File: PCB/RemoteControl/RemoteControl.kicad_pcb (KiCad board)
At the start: 2 copper layers, 44 x 54.5 mm, 14 parts, among them J1 USB_C_Receptacle_USB2.0_14P, J2 Conn_02x05_Top_Bottom, J3 Conn_01x06, J4 Conn_01x03, SW1 SW_Push, U1 STM32L031K6Tx, U2 TC1262-33

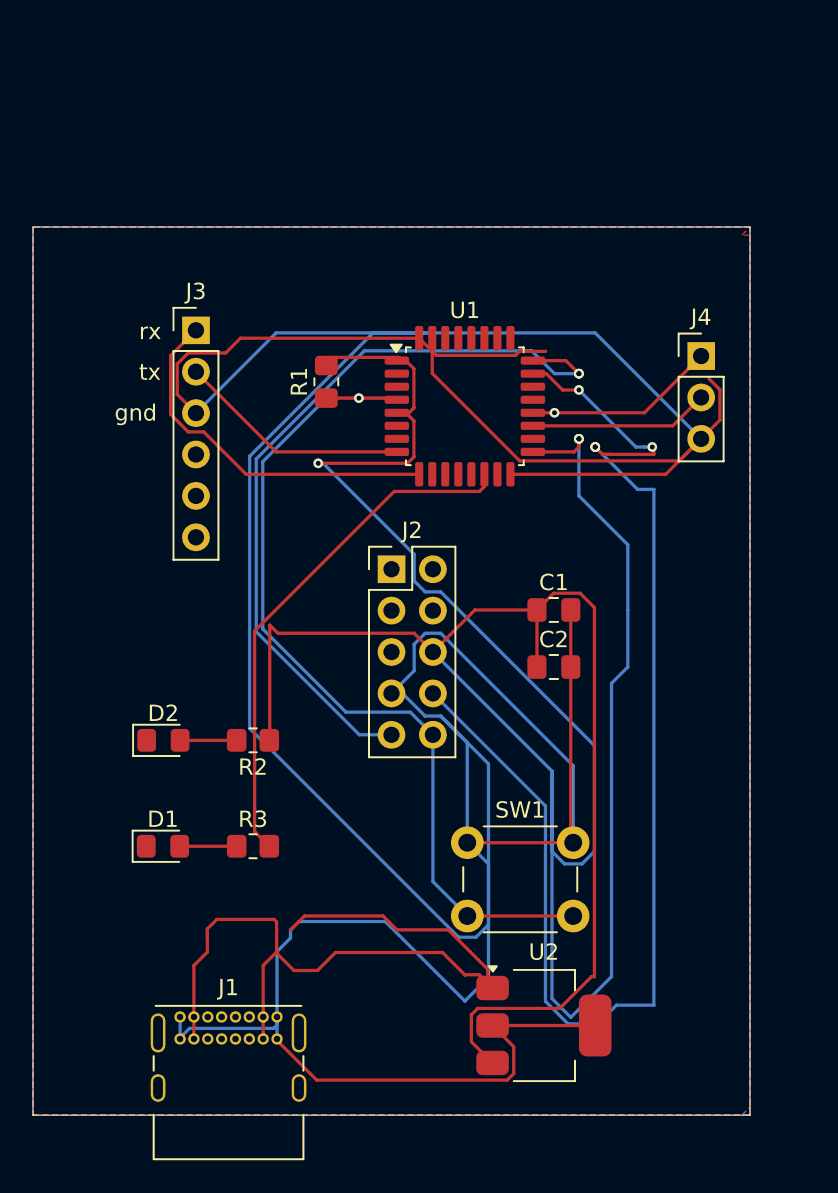
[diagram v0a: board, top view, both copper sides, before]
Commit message: push
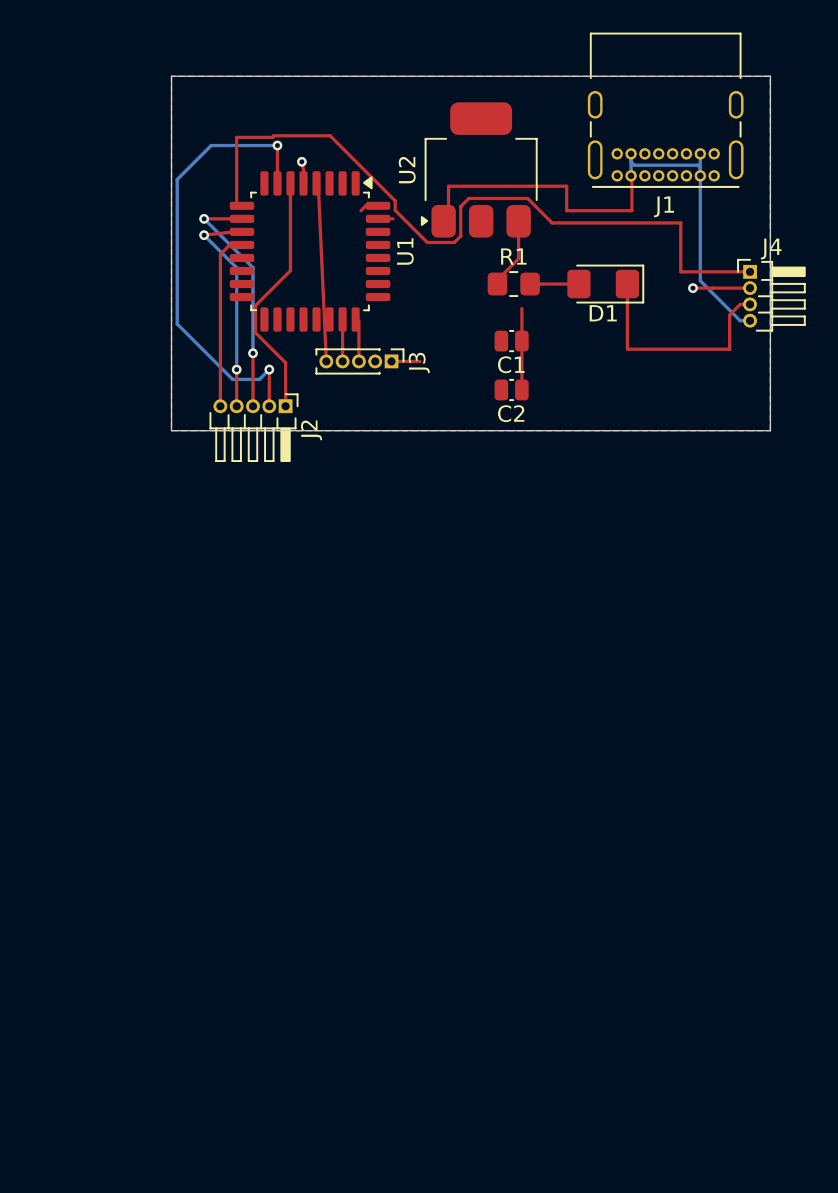
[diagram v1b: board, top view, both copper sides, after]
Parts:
- removed D2: LED, LED_SMD:LED_0805_2012Metric_Pad1.15x1.40mm_HandSolder
- removed R2, R3: 330, Resistor_SMD:R_0805_2012Metric_Pad1.20x1.40mm_HandSolder
- removed SW1: SW_Push, Button_Switch_THT:SW_PUSH_6mm_H4.3mm
- C1: value .1uf -> .1u; footprint Capacitor_SMD:C_0805_2012Metric_Pad1.18x1.45mm_HandSolder -> Capacitor_SMD:C_0504_1310Metric_Pad0.83x1.28mm_HandSolder
- C2: value 10uf -> 1; footprint Capacitor_SMD:C_0805_2012Metric_Pad1.18x1.45mm_HandSolder -> Capacitor_SMD:C_0504_1310Metric_Pad0.83x1.28mm_HandSolder
- D1: footprint LED_SMD:LED_0805_2012Metric_Pad1.15x1.40mm_HandSolder -> LED_SMD:LED_1206_3216Metric_Pad1.42x1.75mm_HandSolder
- J2: value Conn_02x05_Top_Bottom -> Conn_01x05_Socket; footprint Connector_PinHeader_2.54mm:PinHeader_2x05_P2.54mm_Vertical -> Connector_PinHeader_1.00mm:PinHeader_1x05_P1.00mm_Horizontal
- J3: value Conn_01x06 -> Conn_01x05_Pin; footprint Connector_PinHeader_2.54mm:PinHeader_1x06_P2.54mm_Vertical -> Connector_PinHeader_1.00mm:PinHeader_1x05_P1.00mm_Vertical
- J4: value Conn_01x03 -> Conn_01x04_Socket; footprint Connector_PinHeader_2.54mm:PinHeader_1x03_P2.54mm_Vertical -> Connector_PinHeader_1.00mm:PinHeader_1x04_P1.00mm_Horizontal
- R1: value 4.7k -> 270
- moved J1 61.1 mm to (66.3, 25.9), turned to 180 degrees
- moved U2 52.6 mm to (52.0, 25.5), turned to 90 degrees
- moved D1 43.8 mm to (59.5, 32.5), turned to 180 degrees
- moved C2 17.2 mm to (53.9, 39.0), turned to 180 degrees
- moved C1 16.7 mm to (53.9, 36.0), turned to 180 degrees
- moved U1 13.4 mm to (41.5, 30.5), turned to -90 degrees
- moved R1 13.0 mm to (54.0, 32.5), turned to 0 degrees
- moved J3 12.2 mm to (46.5, 37.2), turned to -90 degrees
- moved J2 11.9 mm to (40.0, 40.0), turned to -90 degrees
- moved J4 5.98 mm to (68.5, 31.8)
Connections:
- C1 pad 1: VAPP -> +3.3V
- C2 pad 1: VAPP -> +3.3V
- J2 pad 1: unconnected-(J2-Pin_1-Pad1) -> Finger1
- J2 pad 2: unconnected-(J2-Pin_2-Pad2) -> Finger2
- J2 pad 3: unconnected-(J2-Pin_3-Pad3) -> Finger3
- J2 pad 4: unconnected-(J2-Pin_4-Pad4) -> Finger4
- J2 pad 5: unconnected-(J2-Pin_5-Pad5) -> Finger5
- J3 pad 1: rx -> +3.3V
- J3 pad 2: tx -> GND
- J3 pad 3: GND -> SWSCLK
- J3 pad 4: unconnected-(J3-Pin_4-Pad4) -> SWDIO
- J3 pad 5: unconnected-(J3-Pin_5-Pad5) -> NRST
- J4 pad 1: SDA -> RX
- J4 pad 2: SCL -> TX
- R1 pad 1: NRST -> +3.3V
- R1 pad 2: VAPP -> Net-(D1-A)
- U1 pad 1: VAPP -> +3.3V
- U1 pad 10: unconnected-(U1-PA4-Pad10) -> Finger3
- U1 pad 11: unconnected-(U1-PA5-Pad11) -> Finger4
- U1 pad 12: unconnected-(U1-PA6-Pad12) -> Finger5
- U1 pad 14: Net-(U1-PB0) -> unconnected-(U1-PB0-Pad14)
- U1 pad 17: VAPP -> +3.3V
- U1 pad 19: SCL -> unconnected-(U1-PA9-Pad19)
- U1 pad 20: SDA -> unconnected-(U1-PA10-Pad20)
- U1 pad 23: TMS_SWDIO -> SWDIO
- U1 pad 24: TCK_SWCLK -> SWSCLK
- U1 pad 5: VAPP -> +3.3V
- U1 pad 6: unconnected-(U1-PA0-Pad6) -> Finger1
- U1 pad 7: unconnected-(U1-PA1-Pad7) -> Finger2
- U1 pad 8: tx -> TX
- U1 pad 9: rx -> RX
- U2 pad 3: VAPP -> +3.3V
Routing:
- net GND: track 286.6 -> 16.0 mm
- net VAPP: track 189.8 -> 0.00 mm, vias 3 -> 0
- net TMS_SWDIO: track 79.7 -> 0.00 mm, vias 4 -> 0
- net NRST: track 56.0 -> 0.00 mm, vias 1 -> 0
- net TCK_SWCLK: track 47.8 -> 0.00 mm, vias 2 -> 0
- net Net-(U1-PB0): track 32.1 -> 0.00 mm
- net +5V: track 49.4 -> 18.6 mm
- net RX: track 0.00 -> 30.9 mm
- net Finger2: track 0.00 -> 28.0 mm, vias 0 -> 2
- net rx: track 22.6 -> 0.00 mm
- net Finger1: track 0.00 -> 15.3 mm
- net tx: track 14.4 -> 0.00 mm
- net Finger3: track 0.00 -> 13.0 mm, vias 0 -> 2
- net SDA: track 11.8 -> 0.00 mm, vias 1 -> 0
- net Finger4: track 0.00 -> 11.6 mm, vias 0 -> 2
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- added copper zone on B.Cu, net +3.3V
- removed copper zone on B.Cu, net VAPP
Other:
- board size 44 x 54.5 mm -> 36.8 x 21.8 mm
- board text removed: "gnd"
- board text removed: "rx"
- board text removed: "tx"
